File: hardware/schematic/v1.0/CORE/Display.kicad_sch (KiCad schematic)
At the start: 2 parts, among them U7 FPC-6P

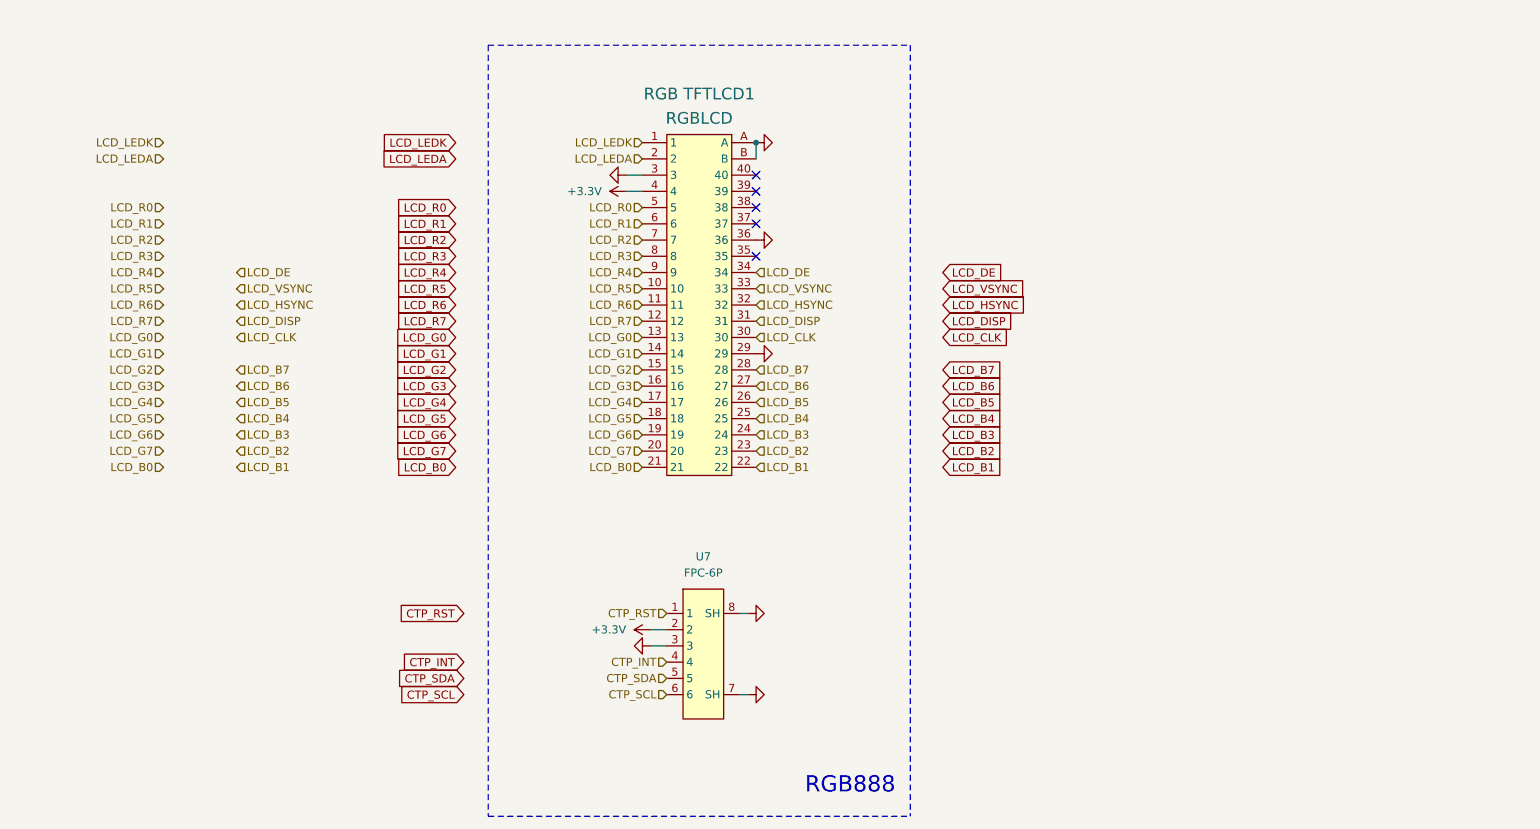
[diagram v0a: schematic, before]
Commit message: sch update
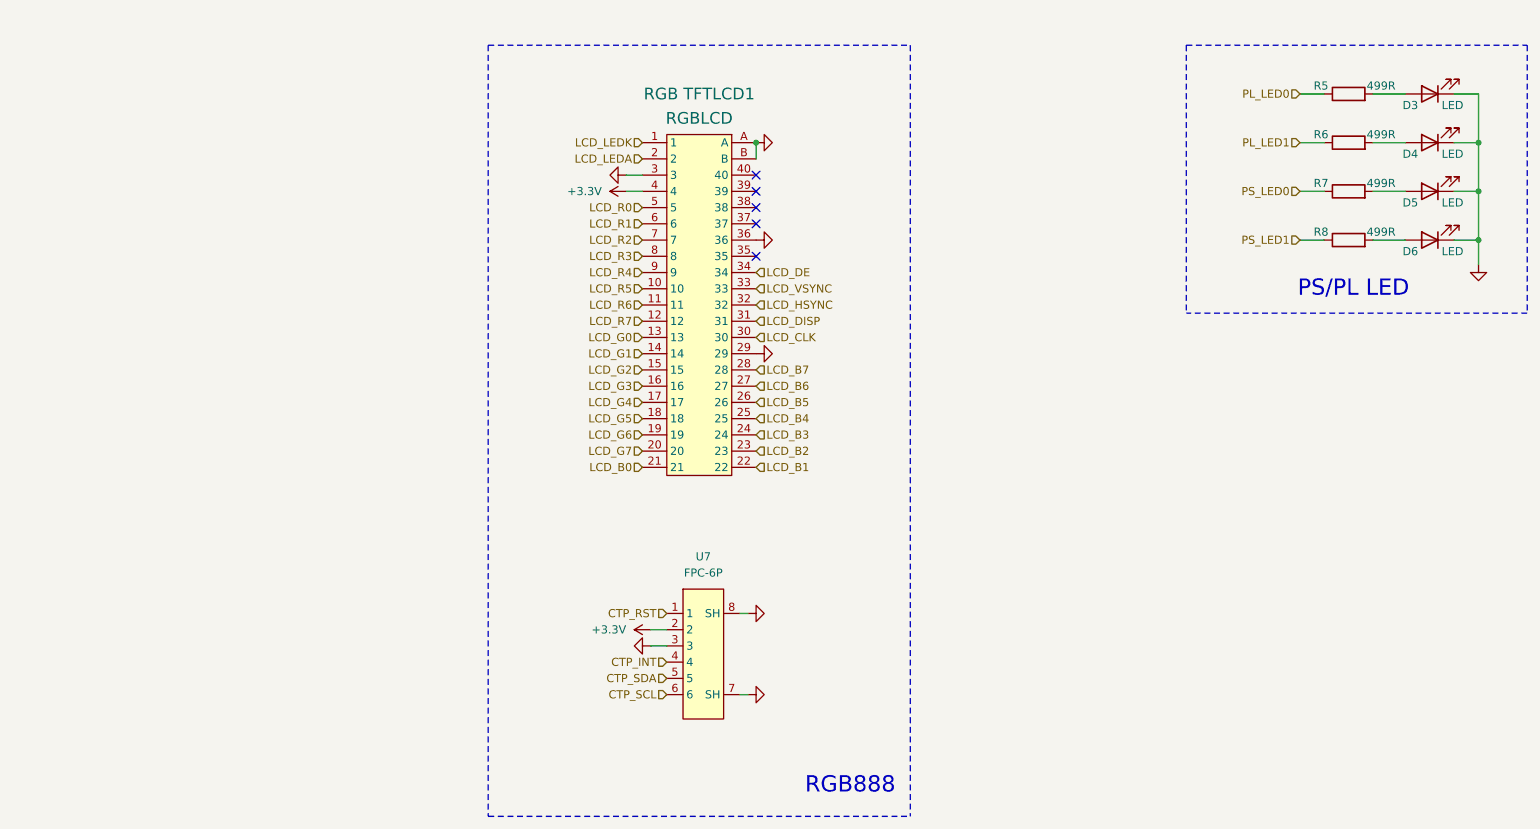
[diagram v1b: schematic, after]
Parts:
- added D3, D4, D5, D6: LED, LED_SMD:LED_0603_1608Metric, symbol Device:LED
- added R5, R6, R7, R8: 499R, Resistor_SMD:R_0402_1005Metric, symbol Device:R
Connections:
- net GND: now also D3.1 (K), D4.1 (K), D5.1 (K), D6.1 (K)
- new net: D6.2 (A), R8.2
- new net: D3.2 (A), R5.2
- new net: D4.2 (A), R6.2
- new net: D5.2 (A), R7.2
- new net PL_LED0: R5.1
- new net PL_LED1: R6.1
- new net PS_LED0: R7.1
- new net PS_LED1: R8.1
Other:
- note added: "PS/PL LED"

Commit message: sch update
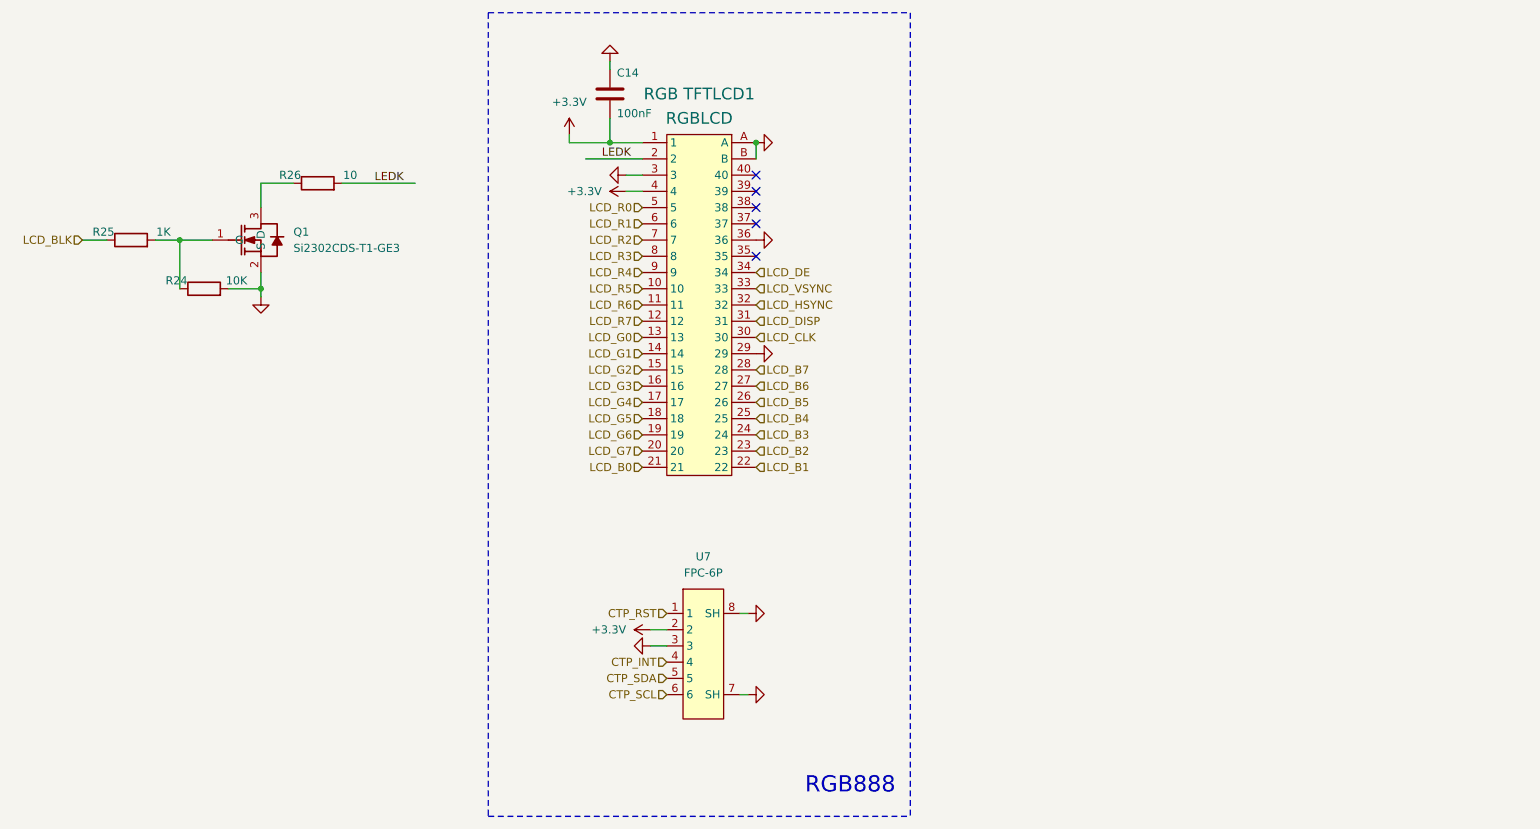
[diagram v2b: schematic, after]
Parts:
- removed D3, D4, D5, D6: LED, LED_SMD:LED_0603_1608Metric, symbol Device:LED
- removed R5, R6, R7, R8: 499R, Resistor_SMD:R_0402_1005Metric, symbol Device:R
- added C14: 100nF, Capacitor_SMD:C_0402_1005Metric, symbol Device:C
- added Q1: Si2302CDS-T1-GE3, JLCImport:Si2302CDS-T1-GE3, symbol JLCImport:Si2302CDS-T1-GE3
- added R24: 10K, Resistor_SMD:R_0402_1005Metric, symbol Device:R
- added R25: 1K, Resistor_SMD:R_0402_1005Metric, symbol Device:R
- added R26: 10, Resistor_SMD:R_0402_1005Metric, symbol Device:R
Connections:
- net LCD_LEDK is gone; now on net +3.3V: RGB TFTLCD1.1
- net +3.3V: now also C14.2
- net GND: now also C14.1, Q1.2 (S), R24.2
- net LCD_LEDA renamed LEDK
- net LEDK: now also R26.2
- new net: Q1.1 (G), R24.1, R25.2
- new net: Q1.3 (D), R26.1
- new net LCD_BLK: R25.1
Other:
- note removed: "PS/PL LED"
